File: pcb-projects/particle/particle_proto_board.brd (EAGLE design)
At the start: 33.7 x 30.5 mm, 35 parts, among them IC1 ATTINY20-MMH, IC2 DMC2400V, IC3 DMC2400V, J2 FTSH-103-XX-XXX-DH, SW1 T/S-PI SW, SW2 T/S-PI SW, SW3 T/S-PI SW

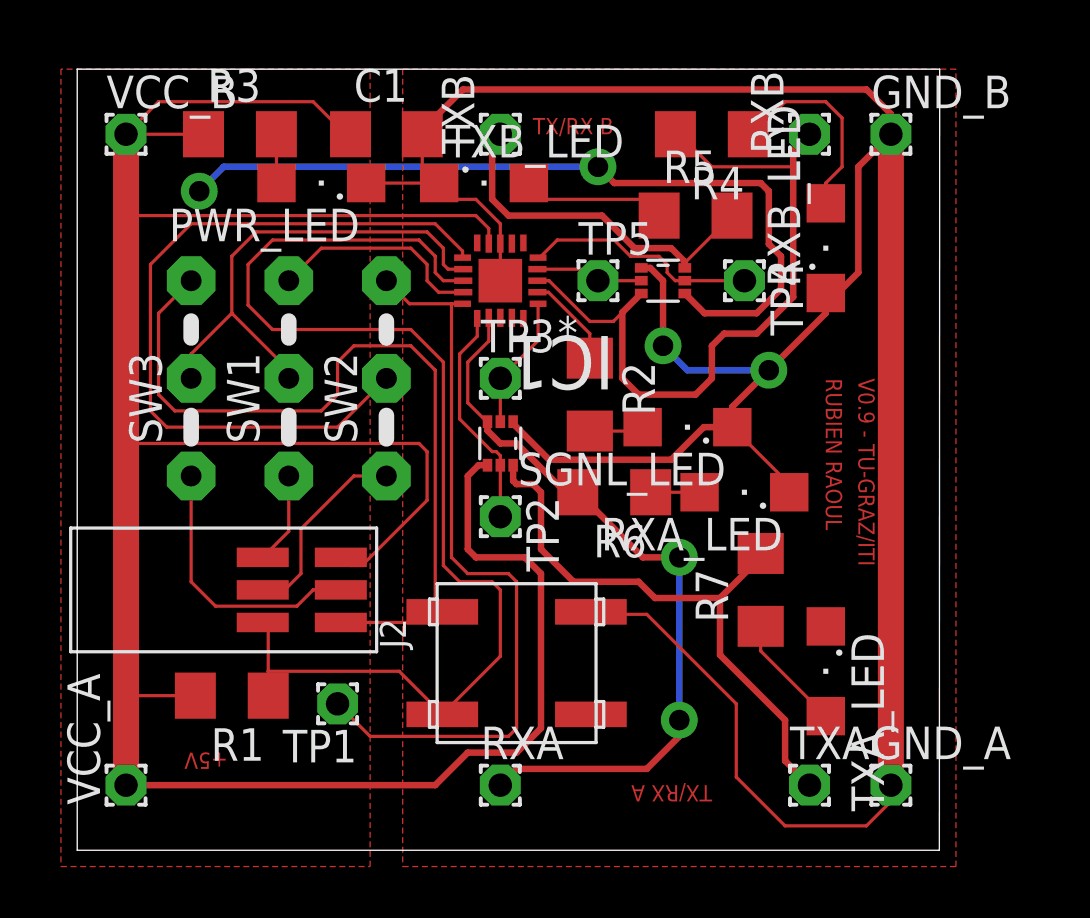
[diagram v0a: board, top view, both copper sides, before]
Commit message: cosmetics
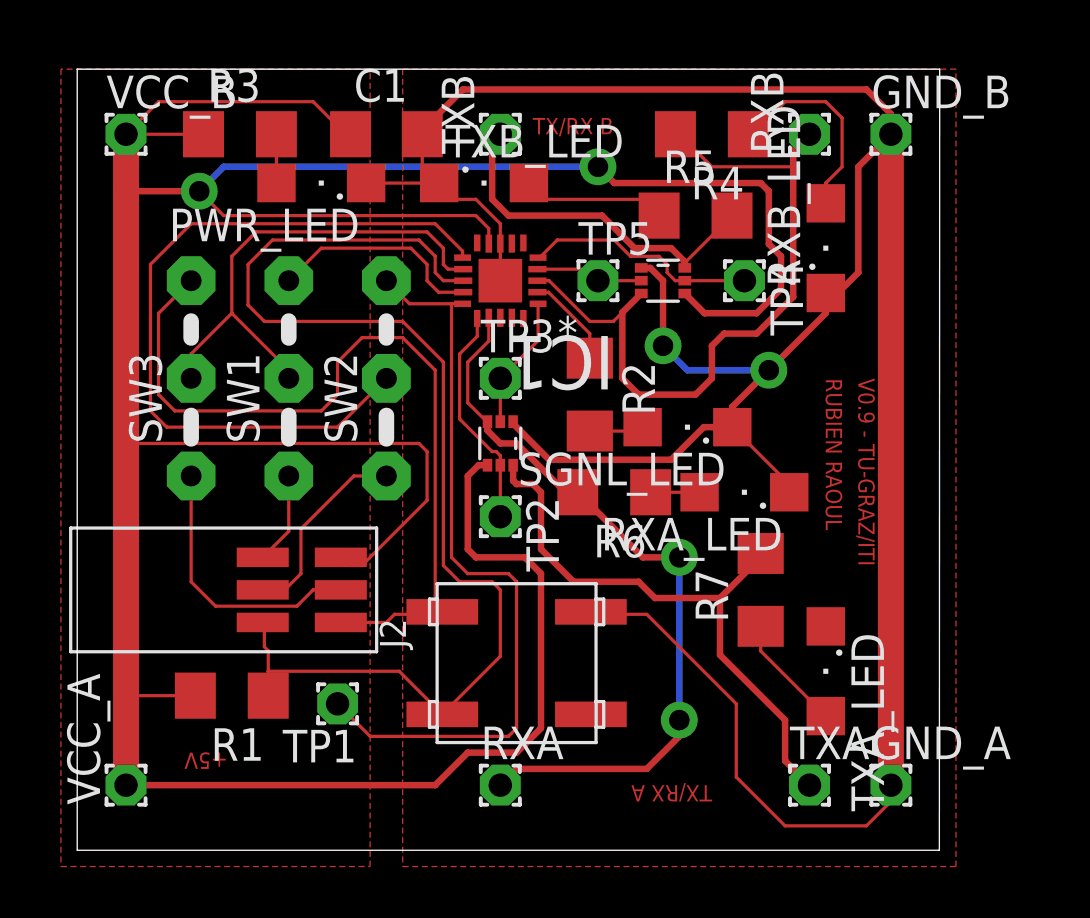
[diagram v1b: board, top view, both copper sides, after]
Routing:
- net GND: track 142.7 -> 143.6 mm
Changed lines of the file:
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@@
 <setting verticaltext="up"/>
 </settings>
-<grid distance="12.5" unitdist="mil" unit="mil" style="lines" multiple="1" display="yes" altdistance="0.00625" altunitdist="inch" altunit="inch"/>
+<grid distance="0.635" unitdist="mm" unit="mm" style="lines" multiple="1" display="yes" altdistance="0.00625" altunitdist="inch" altunit="inch"/>
 <layers>
 <layer number="1" name="Top" color="4" fill="1" visible="yes" active="yes"/>
@@
 <wire x1="10.16" y1="14.605" x2="10.795" y2="15.24" width="0.127" layer="1"/>
 <wire x1="10.795" y1="15.24" x2="10.795" y2="16.51" width="0.127" layer="1"/>
-<wire x1="10.795" y1="16.51" x2="11.43" y2="17.145" width="0.127" layer="1"/>
-<wire x1="11.43" y1="17.145" x2="13.6525" y2="17.145" width="0.127" layer="1"/>
-<wire x1="13.6525" y1="17.145" x2="14.605" y2="16.1925" width="0.127" layer="1"/>
+<wire x1="10.795" y1="16.51" x2="11.7475" y2="17.4625" width="0.127" layer="1"/>
+<wire x1="11.7475" y1="17.4625" x2="13.335" y2="17.4625" width="0.127" layer="1"/>
+<wire x1="13.335" y1="17.4625" x2="14.605" y2="16.1925" width="0.127" layer="1"/>
 <wire x1="14.1" y1="23.845" x2="14.1" y2="25.4" width="0.127" layer="1"/>
 <wire x1="17.145" y1="21.1328" x2="17.145" y2="19.685" width="0.127" layer="1"/>
@@
 <wire x1="14.605" y1="16.1925" x2="14.605" y2="7.0375" width="0.127" layer="1"/>
 <wire x1="14.605" y1="7.0375" x2="14.88" y2="6.7625" width="0.127" layer="1"/>
-<wire x1="10.922" y1="6.35" x2="14.4675" y2="6.35" width="0.127" layer="1"/>
 <wire x1="14.4675" y1="6.35" x2="14.88" y2="6.7625" width="0.127" layer="1"/>
 <wire x1="32.385" y1="0" x2="32.385" y2="-0.635" width="0.127" layer="1"/>
@@
 <wire x1="26.3525" y1="3.175" x2="22.86" y2="6.6675" width="0.127" layer="1"/>
 <wire x1="22.86" y1="6.6675" x2="20.6375" y2="6.6675" width="0.127" layer="1"/>
+<wire x1="10.922" y1="6.35" x2="12.7" y2="6.35" width="0.127" layer="1"/>
+<wire x1="12.7" y1="6.35" x2="13.0175" y2="6.6675" width="0.127" layer="1"/>
+<wire x1="13.0175" y1="6.6675" x2="14.785" y2="6.6675" width="0.127" layer="1"/>
+<wire x1="14.785" y1="6.6675" x2="14.88" y2="6.7625" width="0.127" layer="1"/>
 <wire x1="14.605" y1="16.1925" x2="17.645" y2="14.185" width="0" layer="19" extent="1-1"/>
 </signal>
@@
 <contactref element="R1" pad="1"/>
 <contactref element="IC1" pad="13"/>
-<wire x1="8.255" y1="17.78" x2="13.6525" y2="17.78" width="0.127" layer="1"/>
+<wire x1="7.9375" y1="18.0975" x2="13.335" y2="18.0975" width="0.127" layer="1"/>
 <wire x1="15.6972" y1="19.685" x2="14.9225" y2="19.685" width="0.127" layer="1"/>
 <wire x1="14.9225" y1="19.685" x2="14.605" y2="20.0025" width="0.127" layer="1"/>
@@
 <wire x1="14.605" y1="20.6375" x2="13.97" y2="21.2725" width="0.127" layer="1"/>
 <wire x1="13.97" y1="21.2725" x2="8.255" y2="21.2725" width="0.127" layer="1"/>
-<wire x1="8.255" y1="17.78" x2="7.3025" y2="18.7325" width="0.127" layer="1"/>
+<wire x1="7.9375" y1="18.0975" x2="7.3025" y2="18.7325" width="0.127" layer="1"/>
 <wire x1="7.3025" y1="18.7325" x2="7.3025" y2="20.32" width="0.127" layer="1"/>
 <wire x1="7.3025" y1="20.32" x2="8.255" y2="21.2725" width="0.127" layer="1"/>
-<wire x1="13.6525" y1="17.78" x2="14.9225" y2="16.51" width="0.127" layer="1"/>
+<wire x1="13.335" y1="18.0975" x2="14.9225" y2="16.51" width="0.127" layer="1"/>
 <wire x1="14.9225" y1="16.51" x2="14.9225" y2="8.5725" width="0.127" layer="1"/>
 <contactref element="J2" pad="5"/>
 <contactref element="S2" pad="2"/>
 <wire x1="8.0895" y1="3.4925" x2="8.0895" y2="4.445" width="0.127" layer="1"/>
-<wire x1="8.0895" y1="4.445" x2="8.0895" y2="6.1345" width="0.127" layer="1"/>
 <wire x1="8.0895" y1="6.1345" x2="7.874" y2="6.35" width="0.127" layer="1"/>
 <wire x1="14.9225" y1="8.5725" x2="15.5575" y2="7.9375" width="0.127" layer="1"/>
@@
 <wire x1="13.1975" y1="4.445" x2="8.0895" y2="4.445" width="0.127" layer="1"/>
 <wire x1="8.5725" y1="3.4925" x2="8.0895" y2="3.4925" width="0.127" layer="1"/>
+<wire x1="8.0895" y1="4.445" x2="8.0895" y2="5.2455" width="0.127" layer="1"/>
+<wire x1="8.0895" y1="5.2455" x2="7.9375" y2="5.3975" width="0.127" layer="1"/>
+<wire x1="7.9375" y1="5.3975" x2="7.9375" y2="6.2865" width="0.127" layer="1"/>
+<wire x1="7.9375" y1="6.2865" x2="7.874" y2="6.35" width="0.127" layer="1"/>
 </signal>
 <signal name="RX_B" class="1">
@@
 <wire x1="2.54" y1="25.4" x2="5.563" y2="25.4" width="0.127" layer="1"/>
 <via x="5.3975" y="23.1775" extent="1-16" drill="0.8" shape="square"/>
-<wire x1="16.1925" y1="22.225" x2="2.54" y2="22.225" width="0.127" layer="1"/>
 <wire x1="20.955" y1="24.13" x2="6.35" y2="24.13" width="0.254" layer="16"/>
 <wire x1="6.35" y1="24.13" x2="5.3975" y2="23.1775" width="0.254" layer="16"/>
@@
 <wire x1="2.8575" y1="13.335" x2="2.54" y2="13.6525" width="0.127" layer="1"/>
 <contactref element="J2" pad="2"/>
-<wire x1="5.2455" y1="3.4925" x2="2.8575" y2="3.4925" width="0.127" layer="1"/>
-<wire x1="2.8575" y1="3.4925" x2="2.54" y2="3.81" width="0.127" layer="1"/>
-<wire x1="2.54" y1="25.4" x2="2.54" y2="0" width="1.016" layer="1"/>
+<wire x1="2.54" y1="25.4" x2="2.54" y2="23.1775" width="1.016" layer="1"/>
+<wire x1="2.54" y1="23.1775" x2="2.54" y2="3.81" width="1.016" layer="1"/>
+<wire x1="2.54" y1="3.81" x2="2.54" y2="0" width="1.016" layer="1"/>
 <wire x1="14.2875" y1="11.1125" x2="11.7475" y2="8.5725" width="0.127" layer="1"/>
 <wire x1="11.7475" y1="8.5725" x2="11.2395" y2="8.5725" width="0.127" layer="1"/>
@@
 <wire x1="17.78" y1="1.27" x2="15.875" y2="1.27" width="0.254" layer="1"/>
 <wire x1="15.875" y1="1.27" x2="14.605" y2="0" width="0.254" layer="1"/>
+<wire x1="5.3975" y1="23.1775" x2="2.54" y2="23.1775" width="0.254" layer="1"/>
+<wire x1="16.1925" y1="22.225" x2="6.35" y2="22.225" width="0.127" layer="1"/>
+<wire x1="6.35" y1="22.225" x2="5.3975" y2="23.1775" width="0.127" layer="1"/>
+<wire x1="5.2455" y1="3.4925" x2="2.8575" y2="3.4925" width="0.127" layer="1"/>
+<wire x1="2.8575" y1="3.4925" x2="2.54" y2="3.81" width="0.127" layer="1"/>
 </signal>
 <signal name="TX_B">
